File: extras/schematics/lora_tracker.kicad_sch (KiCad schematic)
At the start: 20 parts, among them J1 Coax, J4 Pwr, SW1 SW_Push, U1 ESP32, U2 E22-400M30S, U3 RA-01, U4 INP441, U5 MAX98357A, U6 SSD1306, U7 KY040

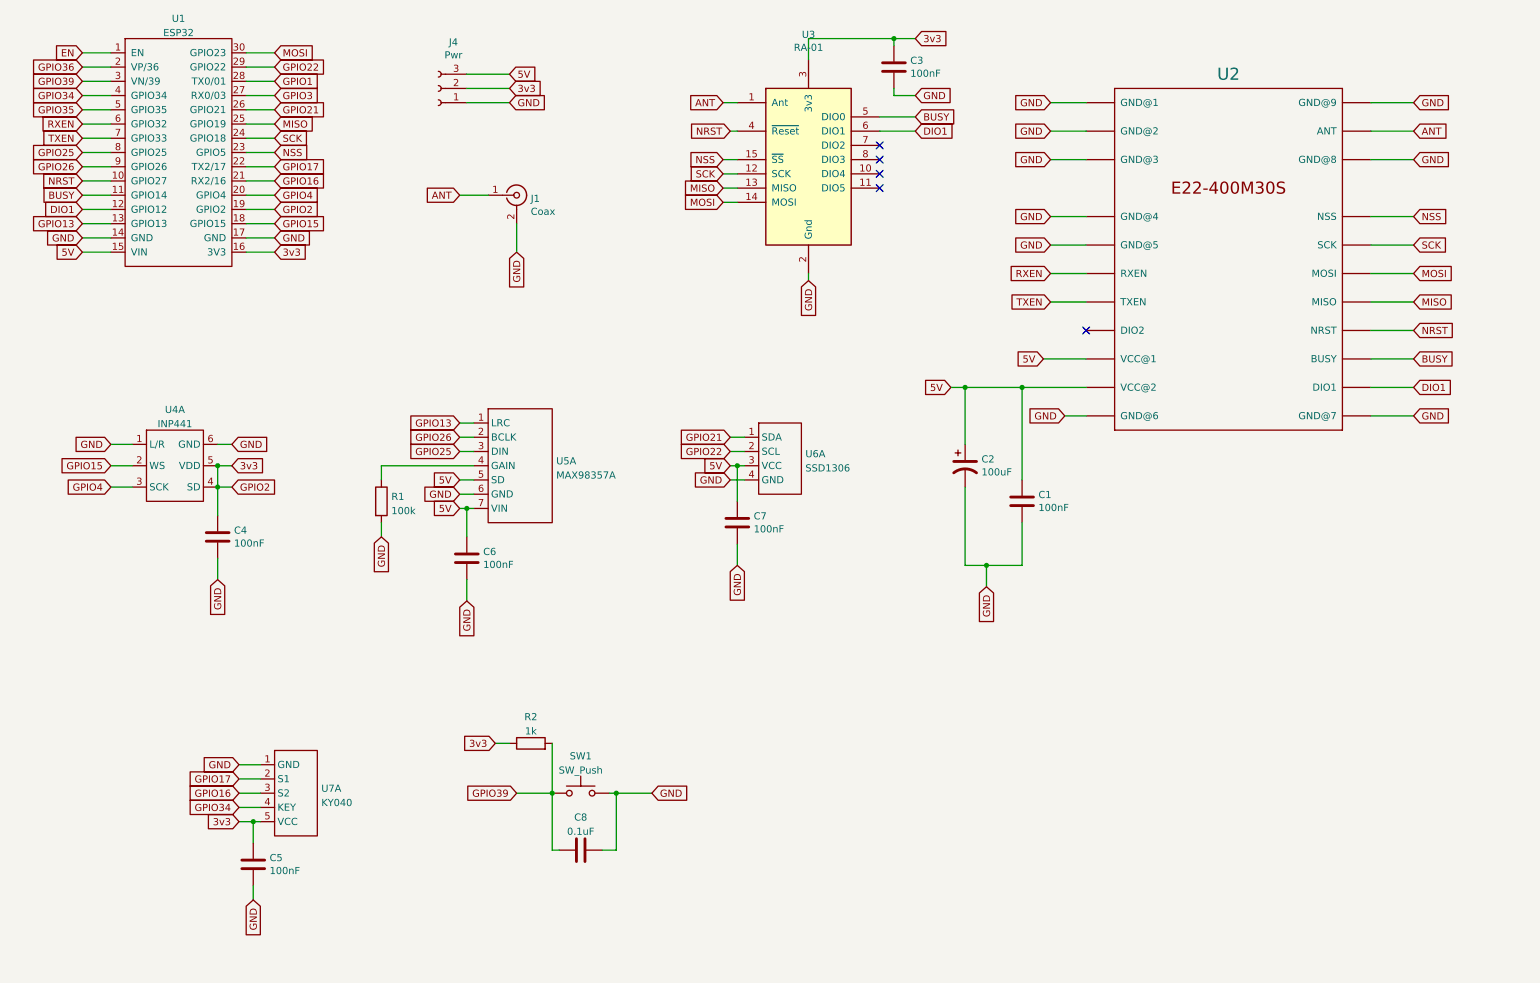
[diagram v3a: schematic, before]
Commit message: Updated schematics
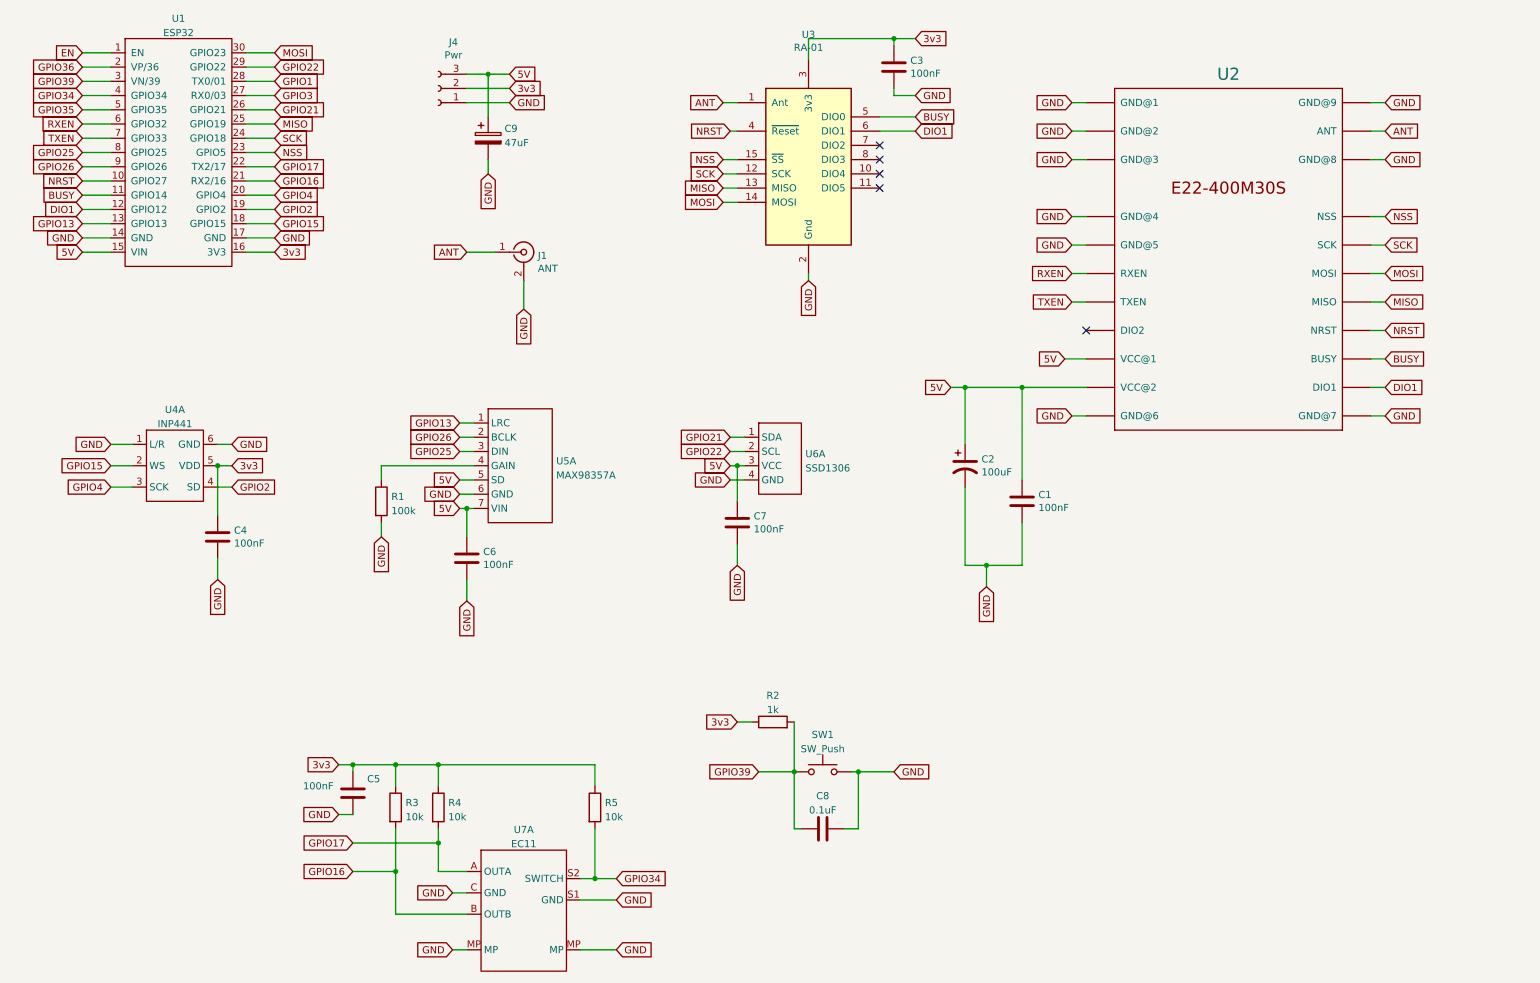
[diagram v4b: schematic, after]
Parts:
- removed U7: KY040, symbol lora_tracker:KY040
- added C9: 47uF, Capacitor_THT:CP_Radial_D4.0mm_P2.00mm, symbol Device:C_Polarized
- added R3, R4, R5: 10k, Resistor_SMD:R_0603_1608Metric_Pad0.98x0.95mm_HandSolder, symbol Device:R
- added U7: EC11, lora_tracker:ec11, symbol lora_tracker:EC11
- J1: value Coax -> ANT
- U1: footprint lora_tracker:esp32-devkit-wide_copy -> lora_tracker:esp32-devkit-wide_30pin
- U4: footprint (none) -> lora_tracker:inp441
- U5: footprint (none) -> lora_tracker:MAX98357A
- U6: footprint (none) -> lora_tracker:SSD1306
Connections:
- net 3v3: now also R3.1, R4.1, R5.1; no longer U1.19 (GPIO2), U4.4 (SD)
- net 5V: now also C9.1
- net GND: now also C9.2, U7.C (GND), U7.MP, U7.S1 (GND)
- net GPIO16: now also R3.2, U7.B (OUTB)
- net GPIO17: now also R4.2, U7.A (OUTA)
- net GPIO34: now also R5.2, U7.S2 (SWITCH)
- new net GPIO2: U1.19 (GPIO2), U4.4 (SD)
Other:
- moved on the sheet: C8, J1, R2, SW1

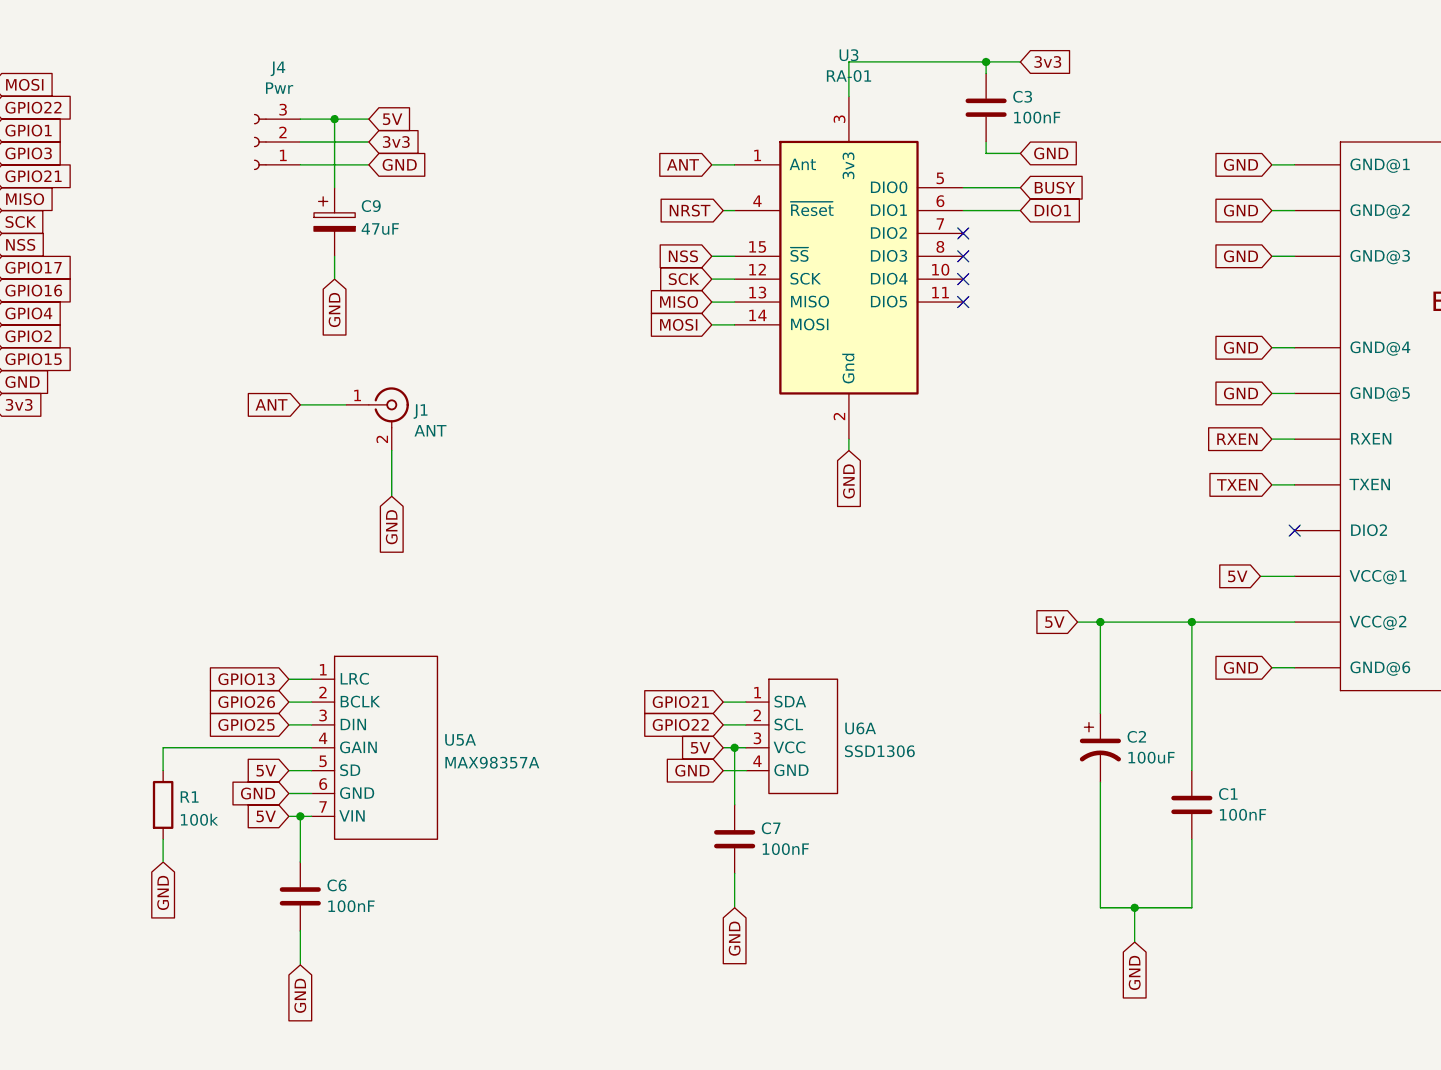
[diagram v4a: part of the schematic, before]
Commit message: Update schematics
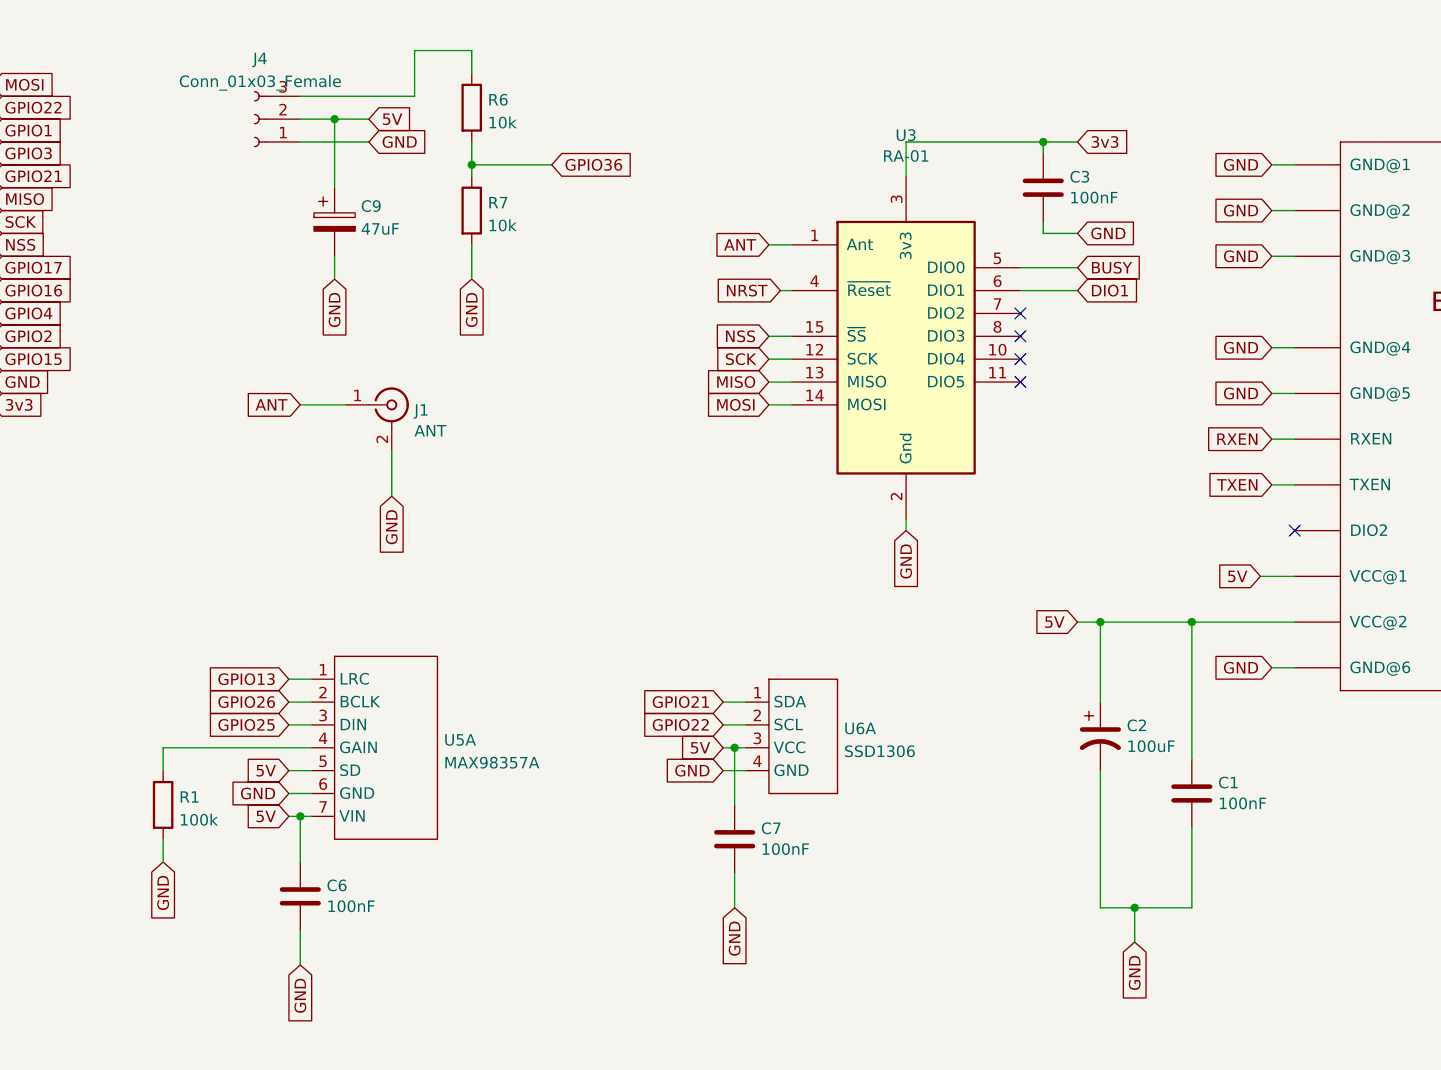
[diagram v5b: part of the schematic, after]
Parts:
- added R6, R7: 10k, Resistor_SMD:R_0603_1608Metric_Pad0.98x0.95mm_HandSolder, symbol Device:R
- J4: value Pwr -> Conn_01x03_Female; footprint Connector_PinSocket_2.54mm:PinSocket_1x03_P2.54mm_Vertical -> Connector_PinHeader_2.54mm:PinHeader_1x03_P2.54mm_Vertical
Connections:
- net 3v3: no longer J4.2 (Pin_2)
- net 5V: now also J4.2 (Pin_2); no longer J4.3 (Pin_3)
- net GND: now also R7.2
- net GPIO36: now also R6.2, R7.1
- new net: J4.3 (Pin_3), R6.1
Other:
- moved on the sheet: C1, C2, C3, U3
